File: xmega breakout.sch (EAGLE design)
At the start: 17 parts, among them IC1 XMEGA16A4A

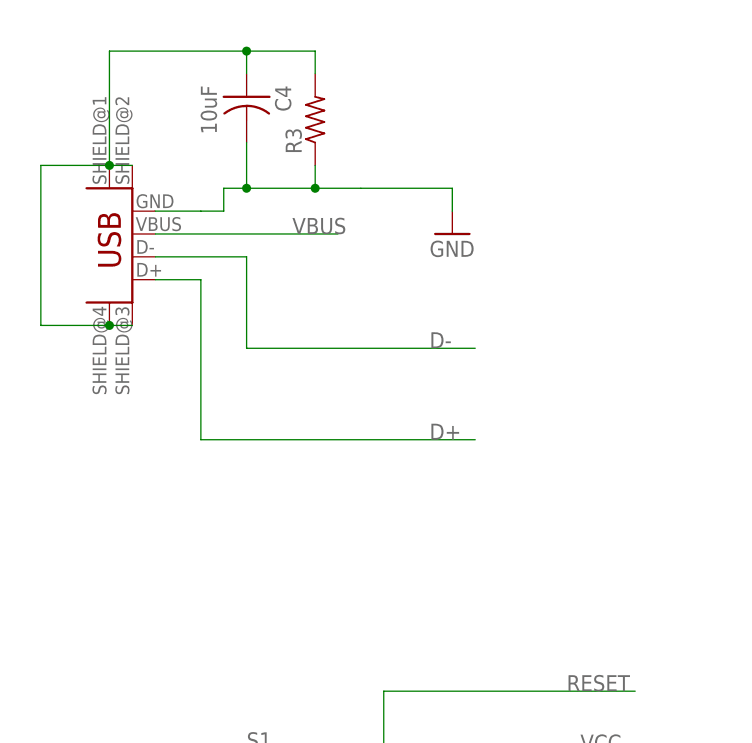
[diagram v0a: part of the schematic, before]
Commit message: typo
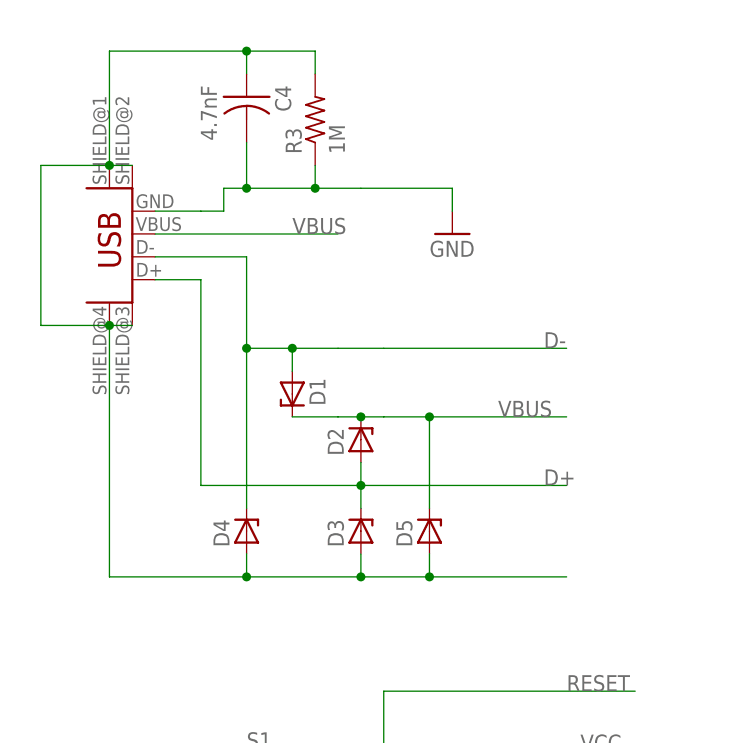
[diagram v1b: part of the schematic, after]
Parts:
- added D1, D2, D3, D4, D5: (no value), fab:ZENER_DIODESOD123
- C4: value 10uF -> 4.7nF
- R3: value (none) -> 1M
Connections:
- net D+: now also D2.ANODE, D3.CATHODE
- net D-: now also D1.ANODE, D4.CATHODE
- net N$25: now also D3.ANODE, D4.ANODE, D5.ANODE
- net VBUS: now also D1.CATHODE, D2.CATHODE, D5.CATHODE
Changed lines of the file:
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@@
 <part name="GND1" library="SparkFun" deviceset="GND" device=""/>
 <part name="P+1" library="SparkFun" deviceset="VCC" device=""/>
-<part name="C4" library="fab" deviceset="CAP-US" device="1206" value="10uF"/>
-<part name="R3" library="fab" deviceset="RES-US" device="1206FAB"/>
+<part name="C4" library="fab" deviceset="CAP-US" device="1206" value="4.7nF"/>
+<part name="R3" library="fab" deviceset="RES-US" device="1206FAB" value="1M"/>
 <part name="GND2" library="SparkFun" deviceset="GND" device=""/>
 <part name="GND3" library="SparkFun" deviceset="GND" device=""/>
@@
 <part name="P+4" library="SparkFun" deviceset="VCC" device=""/>
 <part name="GND5" library="SparkFun" deviceset="GND" device=""/>
+<part name="D1" library="fab" deviceset="ZENER_DIODE" device="SOD123"/>
+<part name="D2" library="fab" deviceset="ZENER_DIODE" device="SOD123"/>
+<part name="D3" library="fab" deviceset="ZENER_DIODE" device="SOD123"/>
+<part name="D4" library="fab" deviceset="ZENER_DIODE" device="SOD123"/>
+<part name="D5" library="fab" deviceset="ZENER_DIODE" device="SOD123"/>
 </parts>
 <sheets>
@@
 <instance part="P+4" gate="1" x="104.14" y="175.26"/>
 <instance part="GND5" gate="1" x="106.68" y="142.24"/>
+<instance part="D1" gate="1" x="-45.72" y="139.7" rot="R270"/>
+<instance part="D2" gate="1" x="-38.1" y="134.62" rot="R90"/>
+<instance part="D3" gate="1" x="-38.1" y="124.46" rot="R90"/>
+<instance part="D4" gate="1" x="-50.8" y="124.46" rot="R90"/>
+<instance part="D5" gate="1" x="-30.48" y="124.46" rot="R90"/>
 </instances>
 <busses>
@@
 <label x="27.94" y="170.18" size="1.778" layer="95"/>
 </segment>
+<segment>
+<wire x1="-45.72" y1="137.16" x2="-40.64" y2="137.16" width="0.1524" layer="91"/>
+<wire x1="-40.64" y1="137.16" x2="-38.1" y2="137.16" width="0.1524" layer="91"/>
+<wire x1="-38.1" y1="137.16" x2="-35.56" y2="137.16" width="0.1524" layer="91"/>
+<wire x1="-35.56" y1="137.16" x2="-30.48" y2="137.16" width="0.1524" layer="91"/>
+<label x="-22.86" y="137.16" size="1.778" layer="95"/>
+<pinref part="D1" gate="1" pin="CATHODE"/>
+<pinref part="D2" gate="1" pin="CATHODE"/>
+<junction x="-38.1" y="137.16"/>
+<pinref part="D5" gate="1" pin="CATHODE"/>
+<wire x1="-30.48" y1="137.16" x2="-15.24" y2="137.16" width="0.1524" layer="91"/>
+<wire x1="-30.48" y1="127" x2="-30.48" y2="137.16" width="0.1524" layer="91"/>
+<junction x="-30.48" y="137.16"/>
+</segment>
 </net>
 <net name="D+" class="0">
@@
 <pinref part="U$1" gate="G$1" pin="D+"/>
 <wire x1="-60.96" y1="152.4" x2="-55.88" y2="152.4" width="0.1524" layer="91"/>
-<wire x1="-55.88" y1="152.4" x2="-55.88" y2="134.62" width="0.1524" layer="91"/>
-<wire x1="-55.88" y1="134.62" x2="-25.4" y2="134.62" width="0.1524" layer="91"/>
-<label x="-30.48" y="134.62" size="1.778" layer="95"/>
+<wire x1="-55.88" y1="152.4" x2="-55.88" y2="129.54" width="0.1524" layer="91"/>
+<wire x1="-55.88" y1="129.54" x2="-38.1" y2="129.54" width="0.1524" layer="91"/>
+<label x="-17.78" y="129.54" size="1.778" layer="95"/>
+<pinref part="D2" gate="1" pin="ANODE"/>
+<wire x1="-38.1" y1="129.54" x2="-15.24" y2="129.54" width="0.1524" layer="91"/>
+<wire x1="-38.1" y1="132.08" x2="-38.1" y2="129.54" width="0.1524" layer="91"/>
+<junction x="-38.1" y="129.54"/>
+<pinref part="D3" gate="1" pin="CATHODE"/>
+<wire x1="-38.1" y1="127" x2="-38.1" y2="129.54" width="0.1524" layer="91"/>
 </segment>
 <segment>
@@
 <wire x1="-60.96" y1="154.94" x2="-50.8" y2="154.94" width="0.1524" layer="91"/>
 <wire x1="-50.8" y1="154.94" x2="-50.8" y2="144.78" width="0.1524" layer="91"/>
-<wire x1="-50.8" y1="144.78" x2="-25.4" y2="144.78" width="0.1524" layer="91"/>
-<label x="-30.48" y="144.78" size="1.778" layer="95"/>
+<wire x1="-50.8" y1="144.78" x2="-45.72" y2="144.78" width="0.1524" layer="91"/>
+<label x="-17.78" y="144.78" size="1.778" layer="95"/>
+<wire x1="-45.72" y1="144.78" x2="-40.64" y2="144.78" width="0.1524" layer="91"/>
+<wire x1="-40.64" y1="144.78" x2="-35.56" y2="144.78" width="0.1524" layer="91"/>
+<wire x1="-35.56" y1="144.78" x2="-15.24" y2="144.78" width="0.1524" layer="91"/>
+<pinref part="D1" gate="1" pin="ANODE"/>
+<wire x1="-45.72" y1="144.78" x2="-45.72" y2="142.24" width="0.1524" layer="91"/>
+<junction x="-45.72" y="144.78"/>
+<pinref part="D4" gate="1" pin="CATHODE"/>
+<wire x1="-50.8" y1="127" x2="-50.8" y2="144.78" width="0.1524" layer="91"/>
+<junction x="-50.8" y="144.78"/>
 </segment>
 <segment>
@@
 <junction x="-50.8" y="177.8"/>
 <wire x1="-73.66" y1="165.1" x2="-66.04" y2="165.1" width="0.1524" layer="91"/>
-</segment>
-</net>
+<wire x1="-66.04" y1="147.32" x2="-66.04" y2="119.38" width="0.1524" layer="91"/>
+<wire x1="-66.04" y1="119.38" x2="-50.8" y2="119.38" width="0.1524" layer="91"/>
+<pinref part="D3" gate="1" pin="ANODE"/>
+<wire x1="-50.8" y1="119.38" x2="-38.1" y2="119.38" width="0.1524" layer="91"/>
+<wire x1="-38.1" y1="119.38" x2="-30.48" y2="119.38" width="0.1524" layer="91"/>
+<wire x1="-30.48" y1="119.38" x2="-15.24" y2="119.38" width="0.1524" layer="91"/>
+<wire x1="-38.1" y1="119.38" x2="-38.1" y2="121.92" width="0.1524" layer="91"/>
+<junction x="-38.1" y="119.38"/>
+<pinref part="D4" gate="1" pin="ANODE"/>
+<wire x1="-50.8" y1="119.38" x2="-50.8" y2="121.92" width="0.1524" layer="91"/>
+<junction x="-50.8" y="119.38"/>
+<pinref part="D5" gate="1" pin="ANODE"/>
+<wire x1="-30.48" y1="119.38" x2="-30.48" y2="121.92" width="0.1524" layer="91"/>
+<junction x="-30.48" y="119.38"/>
+</segment>
+</net>
